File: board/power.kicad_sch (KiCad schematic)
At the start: 9 parts, among them J1 UART, J2 USB_B, U6 FT232RL

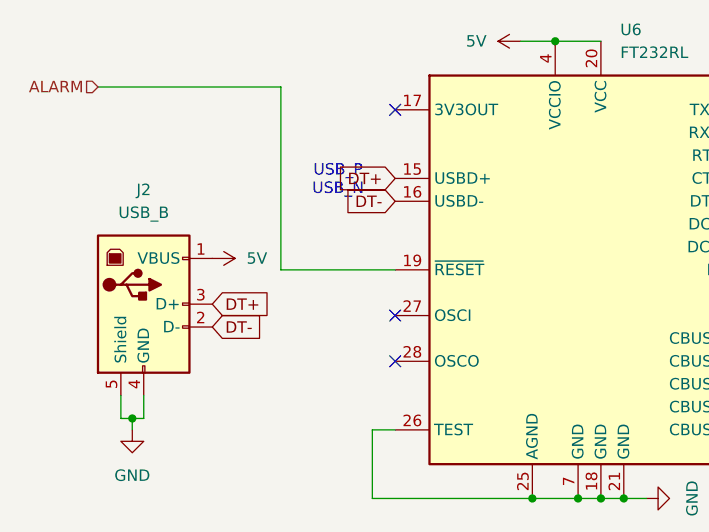
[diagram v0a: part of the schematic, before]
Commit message: add: pcb layout & gerbers
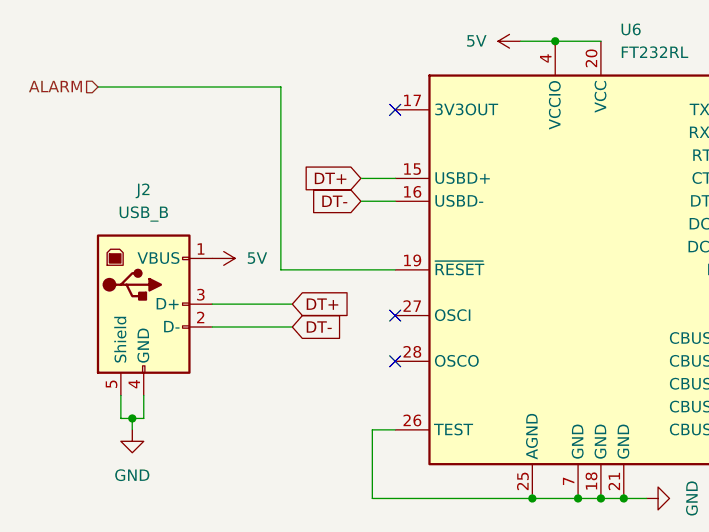
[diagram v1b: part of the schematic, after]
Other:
- note removed: "USB_P USB_N"
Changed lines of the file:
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@@
 	(generator_version "9.0")
 	(paper "User" 177.8 127)
-	(text "USB_P\nUSB_N"
-		(exclude_from_sim no)
-		(at 54.61 35.814 0)
-		(effects
-			(font
-				(size 1.27 1.27)
-			)
-		)
-	)
 	(text_box "Stitching Capacitor"
 		(exclude_from_sim no)
@@
 	(wire
 		(pts
+			(xy 40.64 52.07) (xy 49.53 52.07)
+		)
+		(stroke
+			(width 0)
+			(type default)
+		)
+	)
+	(wire
+		(pts
 			(xy 48.26 45.72) (xy 48.26 25.4)
 		)
@@
 	(wire
 		(pts
+			(xy 40.64 49.53) (xy 49.53 49.53)
+		)
+		(stroke
+			(width 0)
+			(type default)
+		)
+	)
+	(wire
+		(pts
 			(xy 83.82 71.12) (xy 86.36 71.12)
 		)
@@
 		(pts
 			(xy 31.75 62.23) (xy 31.75 63.5)
+		)
+		(stroke
+			(width 0)
+			(type default)
+		)
+	)
+	(wire
+		(pts
+			(xy 57.15 35.56) (xy 60.96 35.56)
+		)
+		(stroke
+			(width 0)
+			(type default)
+		)
+	)
+	(wire
+		(pts
+			(xy 57.15 38.1) (xy 60.96 38.1)
 		)
 		(stroke
@@
 	(global_label "DT-"
 		(shape input)
-		(at 60.96 38.1 180)
+		(at 57.15 38.1 180)
 		(fields_autoplaced yes)
 		(effects
@@
 		)
 		(property "Intersheetrefs" "${INTERSHEET_REFS}"
-			(at 54.1648 38.1 0)
+			(at 50.3548 38.1 0)
 			(effects
 				(font
@@
 	(global_label "DT-"
 		(shape input)
-		(at 40.64 52.07 0)
+		(at 49.53 52.07 0)
 		(fields_autoplaced yes)
 		(effects
@@
 		)
 		(property "Intersheetrefs" "${INTERSHEET_REFS}"
-			(at 47.4352 52.07 0)
+			(at 56.3252 52.07 0)
 			(effects
 				(font
@@
 	(global_label "DT+"
 		(shape input)
-		(at 40.64 49.53 0)
+		(at 49.53 49.53 0)
 		(fields_autoplaced yes)
 		(effects
@@
 		)
 		(property "Intersheetrefs" "${INTERSHEET_REFS}"
-			(at 47.4352 49.53 0)
+			(at 56.3252 49.53 0)
 			(effects
 				(font
@@
 	(global_label "DT+"
 		(shape input)
-		(at 60.96 35.56 180)
+		(at 57.15 35.56 180)
 		(fields_autoplaced yes)
 		(effects
@@
 		)
 		(property "Intersheetrefs" "${INTERSHEET_REFS}"
-			(at 54.1648 35.56 0)
+			(at 50.3548 35.56 0)
 			(effects
 				(font
@@
 		(length 2.54)
 		(shape round)
-		(at 40.64 52.07 0)
-		(fields_autoplaced yes)
-		(effects
-			(font
-				(size 1.27 1.27)
-			)
-			(justify left bottom)
-		)
-		(property "Netclass" "Vias"
-			(at 41.3385 49.53 0)
+		(at 43.18 52.07 180)
+		(fields_autoplaced yes)
+		(effects
+			(font
+				(size 1.27 1.27)
+			)
+			(justify right bottom)
+		)
+		(property "Netclass" "USB"
+			(at 43.8785 54.61 0)
 			(effects
 				(font
@@
 		)
 		(property "Component Class" ""
-			(at -132.08 -59.69 0)
+			(at -129.54 -59.69 0)
 			(effects
 				(font
@@
 		(length 2.54)
 		(shape round)
-		(at 40.64 49.53 0)
+		(at 43.18 49.53 0)
 		(fields_autoplaced yes)
 		(effects
@@
 			(justify left bottom)
 		)
-		(property "Netclass" "Vias"
-			(at 41.3385 46.99 0)
+		(property "Netclass" "USB"
+			(at 43.8785 46.99 0)
 			(effects
 				(font
@@
 		)
 		(property "Component Class" ""
-			(at -132.08 -62.23 0)
-			(effects
-				(font
+			(at -129.54 -62.23 0)
+			(effects
+				(font
